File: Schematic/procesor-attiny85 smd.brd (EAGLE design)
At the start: 27.9 x 27.9 mm, 5 parts

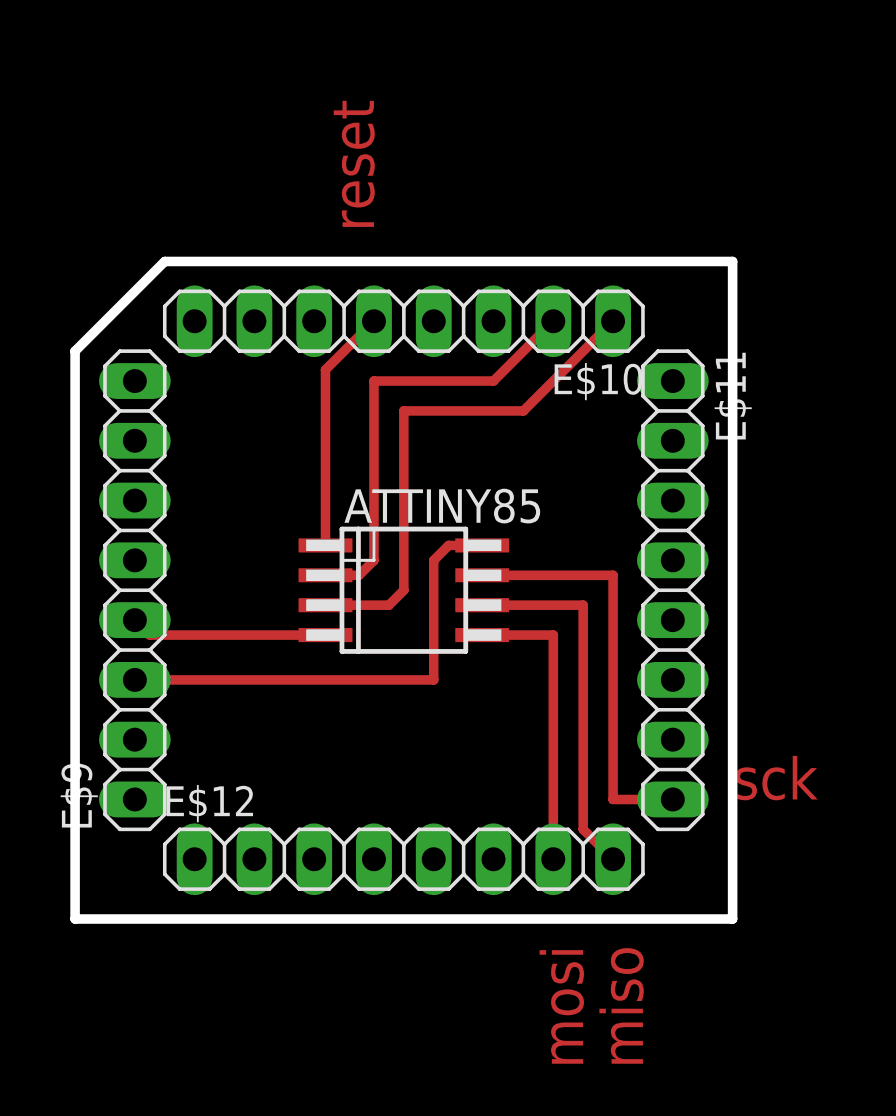
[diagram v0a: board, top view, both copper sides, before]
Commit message: Add files via upload
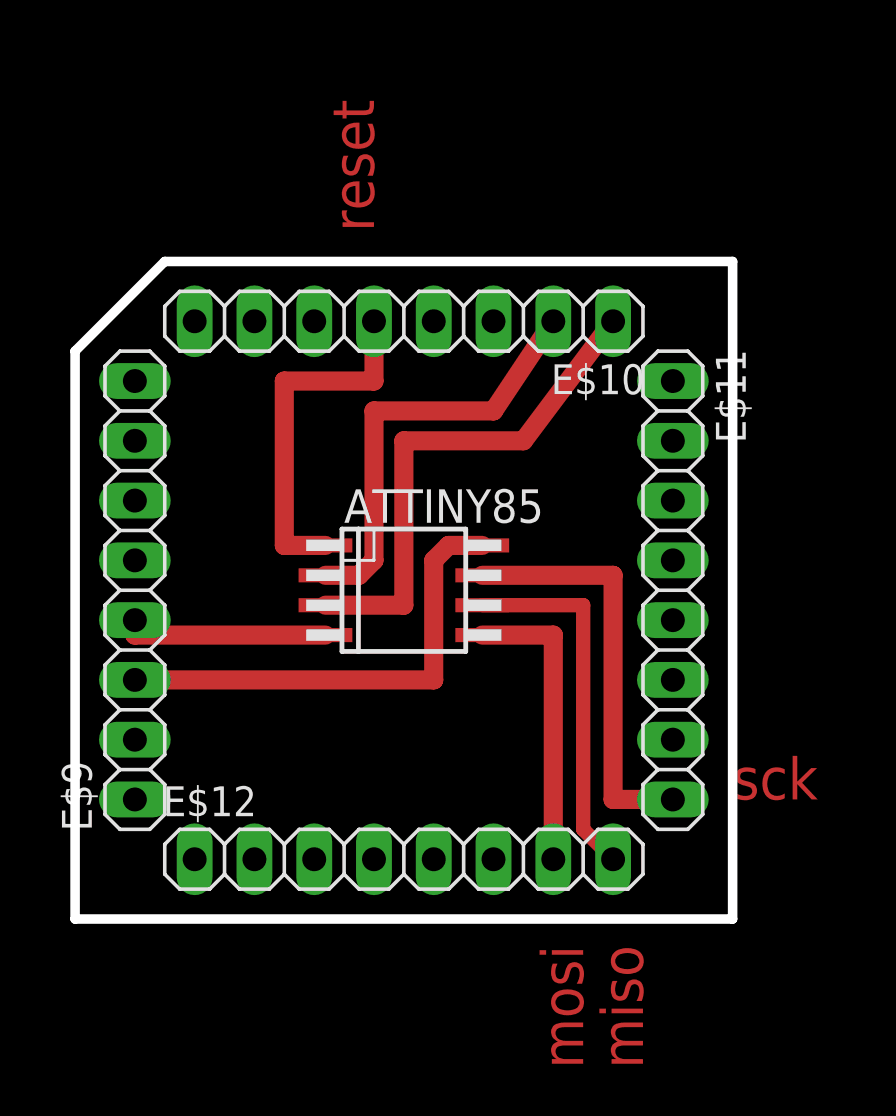
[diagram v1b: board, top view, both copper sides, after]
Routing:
- net S$2: track 10.4 -> 15.1 mm
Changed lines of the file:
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@@
 <setting verticaltext="up"/>
 </settings>
-<grid distance="0.05" unitdist="inch" unit="inch" style="lines" multiple="1" display="yes" altdistance="0.025" altunitdist="inch" altunit="inch"/>
+<grid distance="0.05" unitdist="inch" unit="mm" style="lines" multiple="1" display="yes" altdistance="0.025" altunitdist="inch" altunit="inch"/>
 <layers>
 <layer number="1" name="Top" color="4" fill="1" visible="yes" active="yes"/>
@@
 <contactref element="ATTINY85" pad="1"/>
 <contactref element="E$10" pad="5"/>
-<wire x1="-3.33" y1="1.905" x2="-3.33" y2="9.37" width="0.4064" layer="1"/>
-<wire x1="-3.33" y1="9.37" x2="-1.27" y2="11.43" width="0.4064" layer="1"/>
+<wire x1="-3.33" y1="1.905" x2="-5.08" y2="1.905" width="0.8128" layer="1"/>
+<wire x1="-5.08" y1="1.905" x2="-5.08" y2="8.89" width="0.8128" layer="1"/>
+<wire x1="-5.08" y1="8.89" x2="-1.27" y2="8.89" width="0.8128" layer="1"/>
+<wire x1="-1.27" y1="8.89" x2="-1.27" y2="11.43" width="0.8128" layer="1"/>
 </signal>
 <signal name="S$3">
 <contactref element="E$9" pad="4"/>
 <contactref element="ATTINY85" pad="4"/>
-<wire x1="-3.33" y1="-1.905" x2="-10.795" y2="-1.905" width="0.4064" layer="1"/>
-<wire x1="-10.795" y1="-1.905" x2="-11.43" y2="-1.27" width="0.4064" layer="1"/>
+<wire x1="-3.33" y1="-1.905" x2="-11.43" y2="-1.905" width="0.8128" layer="1"/>
+<wire x1="-11.43" y1="-1.905" x2="-11.43" y2="-1.27" width="0.8128" layer="1"/>
 </signal>
 <signal name="S$4">
 <contactref element="E$9" pad="3"/>
 <contactref element="ATTINY85" pad="8"/>
-<wire x1="3.33" y1="1.905" x2="1.905" y2="1.905" width="0.4064" layer="1"/>
-<wire x1="1.905" y1="1.905" x2="1.27" y2="1.27" width="0.4064" layer="1"/>
-<wire x1="1.27" y1="1.27" x2="1.27" y2="-3.81" width="0.4064" layer="1"/>
-<wire x1="1.27" y1="-3.81" x2="-11.43" y2="-3.81" width="0.4064" layer="1"/>
+<wire x1="1.905" y1="1.905" x2="1.27" y2="1.27" width="0.8128" layer="1"/>
+<wire x1="1.27" y1="1.27" x2="1.27" y2="-3.81" width="0.8128" layer="1"/>
+<wire x1="1.27" y1="-3.81" x2="-11.43" y2="-3.81" width="0.8128" layer="1"/>
+<wire x1="1.905" y1="1.905" x2="3.33" y2="1.905" width="0.8128" layer="1"/>
 </signal>
 <signal name="S$6">
 <contactref element="E$10" pad="1"/>
 <contactref element="ATTINY85" pad="3"/>
-<wire x1="-3.33" y1="-0.635" x2="-0.635" y2="-0.635" width="0.4064" layer="1"/>
-<wire x1="-0.635" y1="-0.635" x2="0" y2="0" width="0.4064" layer="1"/>
-<wire x1="0" y1="0" x2="0" y2="7.62" width="0.4064" layer="1"/>
-<wire x1="0" y1="7.62" x2="5.08" y2="7.62" width="0.4064" layer="1"/>
-<wire x1="5.08" y1="7.62" x2="8.89" y2="11.43" width="0.4064" layer="1"/>
+<wire x1="-3.33" y1="-0.635" x2="0" y2="-0.635" width="0.8128" layer="1"/>
+<wire x1="0" y1="-0.635" x2="0" y2="6.35" width="0.8128" layer="1"/>
+<wire x1="0" y1="6.35" x2="5.08" y2="6.35" width="0.8128" layer="1"/>
+<wire x1="5.08" y1="6.35" x2="8.89" y2="11.43" width="0.8128" layer="1"/>
 </signal>
 <signal name="S$7">
 <contactref element="E$10" pad="2"/>
 <contactref element="ATTINY85" pad="2"/>
-<wire x1="-3.33" y1="0.635" x2="-1.905" y2="0.635" width="0.4064" layer="1"/>
-<wire x1="-1.905" y1="0.635" x2="-1.27" y2="1.27" width="0.4064" layer="1"/>
-<wire x1="-1.27" y1="1.27" x2="-1.27" y2="8.89" width="0.4064" layer="1"/>
-<wire x1="-1.27" y1="8.89" x2="3.81" y2="8.89" width="0.4064" layer="1"/>
-<wire x1="3.81" y1="8.89" x2="6.35" y2="11.43" width="0.4064" layer="1"/>
+<wire x1="6.35" y1="11.43" x2="3.81" y2="7.62" width="0.8128" layer="1"/>
+<wire x1="3.81" y1="7.62" x2="-1.27" y2="7.62" width="0.8128" layer="1"/>
+<wire x1="-1.27" y1="7.62" x2="-1.27" y2="1.27" width="0.8128" layer="1"/>
+<wire x1="-1.27" y1="1.27" x2="-1.905" y2="0.635" width="0.8128" layer="1"/>
+<wire x1="-1.905" y1="0.635" x2="-3.33" y2="0.635" width="0.8128" layer="1"/>
 </signal>
 <signal name="S$5">
 <contactref element="E$11" pad="8"/>
 <contactref element="ATTINY85" pad="7"/>
-<wire x1="3.33" y1="0.635" x2="8.89" y2="0.635" width="0.4064" layer="1"/>
-<wire x1="8.89" y1="0.635" x2="8.89" y2="-8.89" width="0.4064" layer="1"/>
-<wire x1="8.89" y1="-8.89" x2="11.43" y2="-8.89" width="0.4064" layer="1"/>
+<wire x1="3.33" y1="0.635" x2="8.89" y2="0.635" width="0.8128" layer="1"/>
+<wire x1="8.89" y1="0.635" x2="8.89" y2="-8.89" width="0.8128" layer="1"/>
+<wire x1="8.89" y1="-8.89" x2="11.43" y2="-8.89" width="0.8128" layer="1"/>
 </signal>
 <signal name="S$8">
 <contactref element="E$12" pad="7"/>
 <contactref element="ATTINY85" pad="5"/>
-<wire x1="3.33" y1="-1.905" x2="6.35" y2="-1.905" width="0.4064" layer="1"/>
-<wire x1="6.35" y1="-1.905" x2="6.35" y2="-11.43" width="0.4064" layer="1"/>
+<wire x1="3.33" y1="-1.905" x2="6.35" y2="-1.905" width="0.8128" layer="1"/>
+<wire x1="6.35" y1="-1.905" x2="6.35" y2="-11.43" width="0.8128" layer="1"/>
 </signal>
 <signal name="S$10">
 <contactref element="E$12" pad="8"/>
 <contactref element="ATTINY85" pad="6"/>
-<wire x1="3.33" y1="-0.635" x2="7.62" y2="-0.635" width="0.4064" layer="1"/>
-<wire x1="7.62" y1="-0.635" x2="7.62" y2="-10.16" width="0.4064" layer="1"/>
-<wire x1="7.62" y1="-10.16" x2="8.89" y2="-11.43" width="0.4064" layer="1"/>
+<wire x1="8.89" y1="-11.43" x2="7.62" y2="-10.16" width="0.6096" layer="1"/>
+<wire x1="7.62" y1="-10.16" x2="7.62" y2="-0.635" width="0.6096" layer="1"/>
+<wire x1="7.62" y1="-0.635" x2="3.33" y2="-0.635" width="0.6096" layer="1"/>
 </signal>
 </signals>
